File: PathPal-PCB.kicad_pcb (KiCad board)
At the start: 4 copper layers, 110 x 40 mm, 36 parts, among them J1 Raspberry_Pi_2_3, J2 Motor, J3 Button1, J4 Button2, J5 Button3, J6 Motor, Q1 AO3400A, Q2 AO3400A, Q3 AO3400A, Q4 AO3400A, U1 Gyro, U2 HR, U3 LiDAR

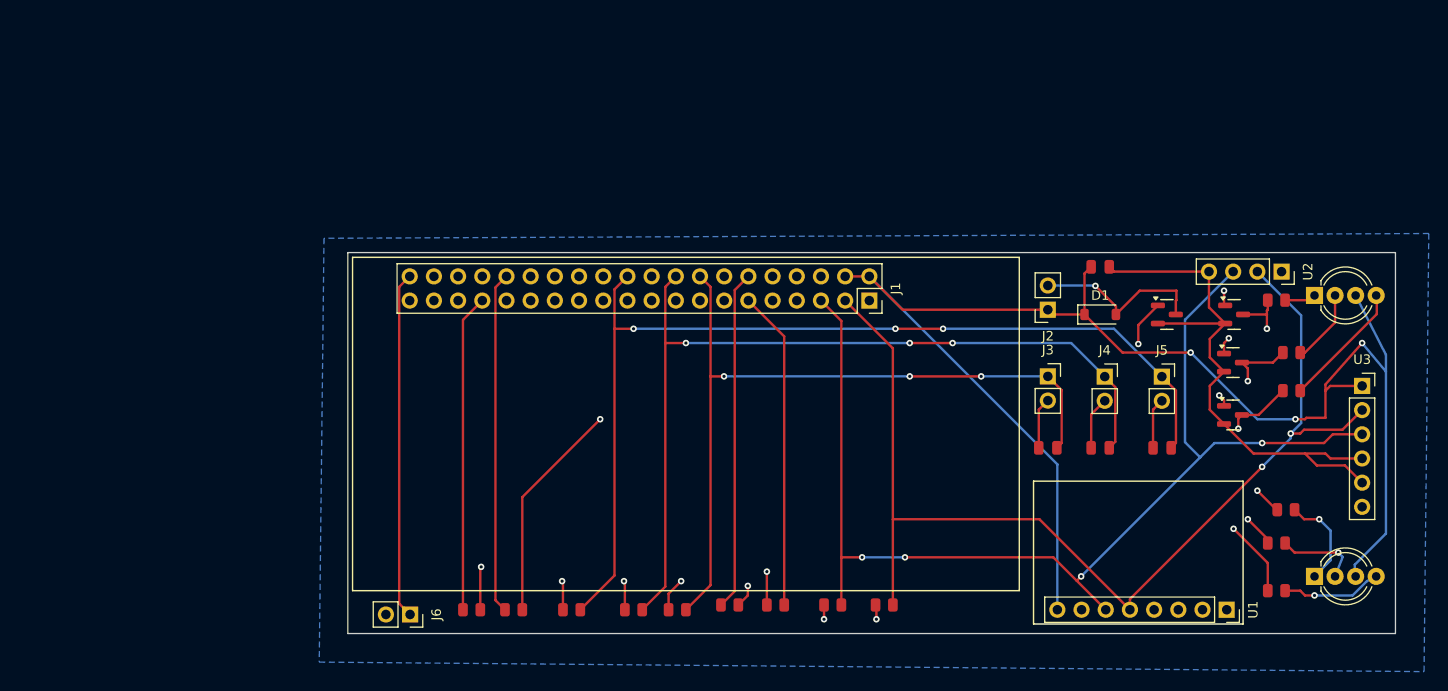
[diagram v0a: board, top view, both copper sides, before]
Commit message: simpler
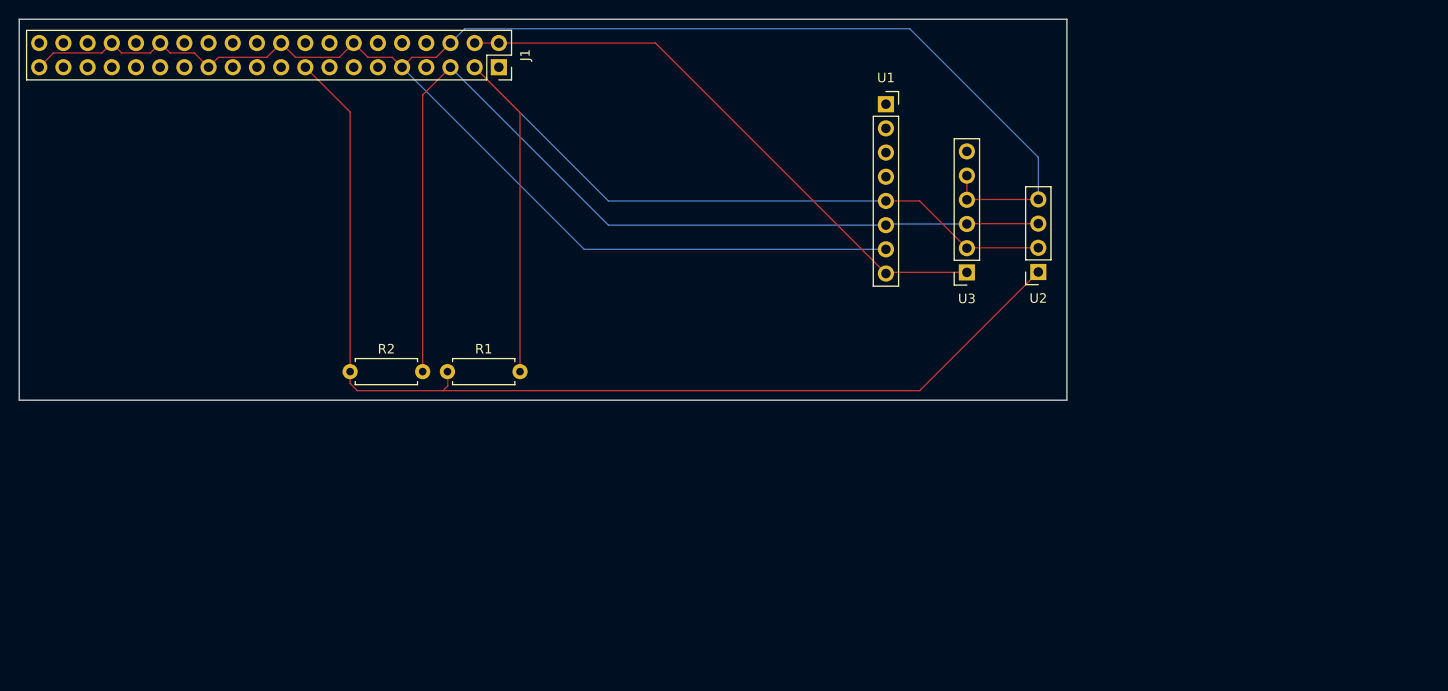
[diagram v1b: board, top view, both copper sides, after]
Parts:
- removed C1: 10uF, PCM_JLCPCB:C_0805
- removed C2, C3, C4: 100nF, PCM_JLCPCB:C_0805
- removed D1: 1N4148W, Diode_SMD:D_SOD-123
- removed D2, D3: LED_RGAB, LED_THT:LED_D5.0mm-4_RGB_Wide_Pins
- removed G***: LOGO, LOGO
- removed J2, J6: Motor, Connector_PinSocket_2.54mm:PinSocket_1x02_P2.54mm_Vertical
- removed J3: Button1, Connector_PinSocket_2.54mm:PinSocket_1x02_P2.54mm_Vertical
- removed J4: Button2, Connector_PinSocket_2.54mm:PinSocket_1x02_P2.54mm_Vertical
- removed J5: Button3, Connector_PinSocket_2.54mm:PinSocket_1x02_P2.54mm_Vertical
- removed Q1, Q2, Q3, Q4: AO3400A, PCM_JLCPCB:Q_SOT-23
- removed R10, R15, R9: 10kΩ, PCM_JLCPCB:R_0805
- removed R11, R12, R13, R14: 100Ω, PCM_JLCPCB:R_0805
- removed R3, R4, R5, R6: 1kΩ, PCM_JLCPCB:R_0805
- removed R7, R8: 150Ω, PCM_JLCPCB:R_0805
- R1, R2: footprint PCM_JLCPCB:R_0805 -> Resistor_THT:R_Axial_DIN0207_L6.3mm_D2.5mm_P7.62mm_Horizontal
- moved U1 64.0 mm to (141.5, 48.9), turned to 0 degrees
- moved R2 56.3 mm to (85.2, 77.0)
- moved R1 52.0 mm to (95.5, 77.0)
- moved J1 46.0 mm to (100.9, 45.0)
- moved U3 43.2 mm to (150.0, 66.6), turned to 180 degrees
- moved U2 25.5 mm to (157.5, 66.5), turned to 180 degrees
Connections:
- J1 pad 11: /MotorSEL -> unconnected-(J1-GPIO17-Pad11)
- J1 pad 12: /BLedSEL -> unconnected-(J1-GPIO18/PWM0-Pad12)
- J1 pad 16: /Button1IN -> unconnected-(J1-GPIO23-Pad16)
- J1 pad 18: /Button2IN -> unconnected-(J1-GPIO24-Pad18)
- J1 pad 22: /Button3IN -> unconnected-(J1-GPIO25-Pad22)
- J1 pad 32: /RLedSEL -> unconnected-(J1-PWM0/GPIO12-Pad32)
- J1 pad 33: /GLedSEL -> unconnected-(J1-PWM1/GPIO13-Pad33)
- J1 pad 40: /BatLow -> unconnected-(J1-GPIO21/SCLK1-Pad40)
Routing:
- net GND: track 76.4 -> 191.7 mm
- net /Button3IN: track 104.9 -> 0.00 mm, vias 3 -> 0
- net Net-(Q2-G): track 96.1 -> 0.00 mm, vias 2 -> 0
- net Net-(Q3-G): track 94.8 -> 0.00 mm, vias 2 -> 0
- net +5V: track 154.1 -> 61.8 mm, vias 3 -> 0
- net /Button2IN: track 92.3 -> 0.00 mm, vias 3 -> 0
- net /Button1IN: track 80.3 -> 0.00 mm, vias 3 -> 0
- net +3.3V: track 47.3 -> 115.1 mm, vias 5 -> 0
- net Net-(Q4-G): track 61.5 -> 0.00 mm, vias 2 -> 0
- net Net-(Q1-G): track 57.3 -> 0.00 mm, vias 2 -> 0
- net /BatLow: track 36.4 -> 0.00 mm
- net /RLedSEL: track 35.9 -> 0.00 mm
- net /BLedSEL: track 35.7 -> 0.00 mm
- net /MotorSEL: track 33.5 -> 0.00 mm
- net /GLedSEL: track 33.3 -> 0.00 mm
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- removed copper zone on In2.Cu, net +3.3V
- removed copper zone on B.Cu, net GND
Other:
- board text removed: "JLCJLCJLCJLC"
- board text removed: "Pathpal Senseway V2.0"
